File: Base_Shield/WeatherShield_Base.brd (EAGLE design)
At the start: 67.3 x 58.4 mm, 68 parts, among them Q1 BSS138, Q2 BSS138, U1 DS3231SN, U2 LT3652, U3 TMP100MDBVREP, U4 ADS1015IDGST

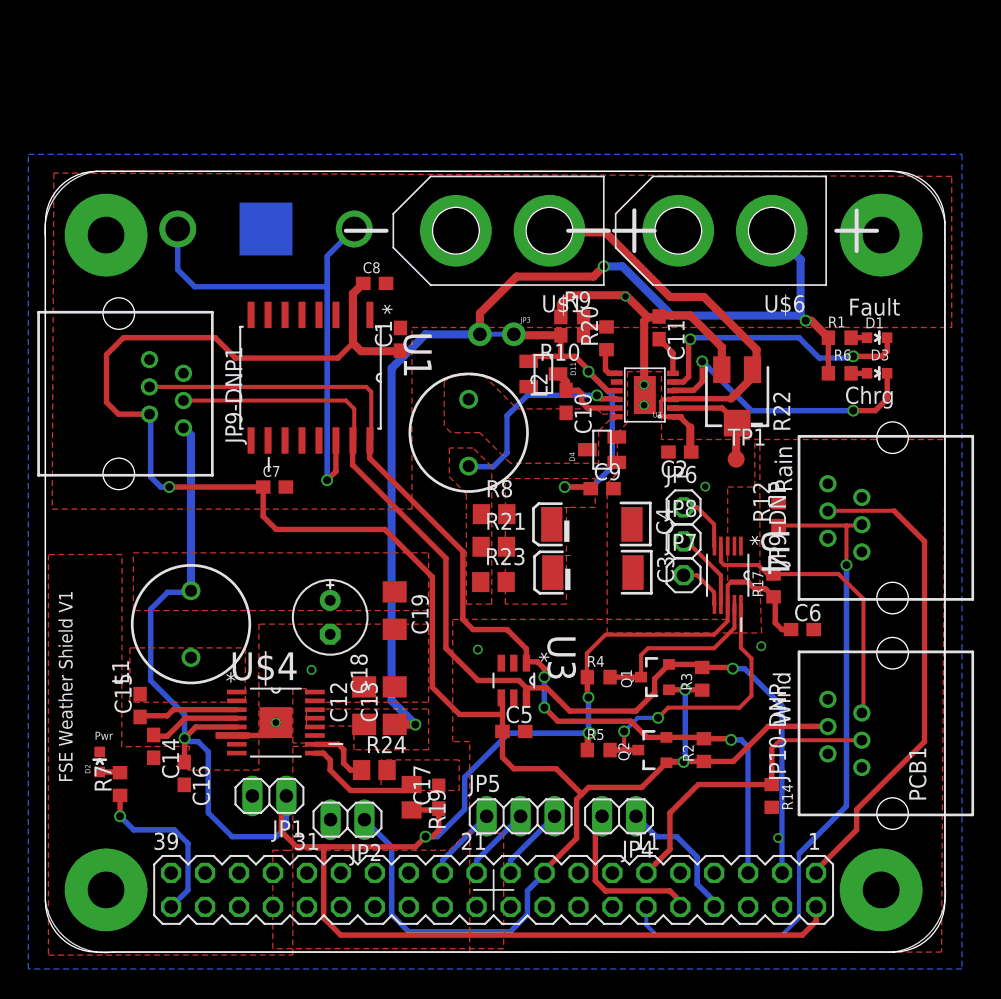
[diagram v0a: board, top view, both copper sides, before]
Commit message: WeatherShield_v1
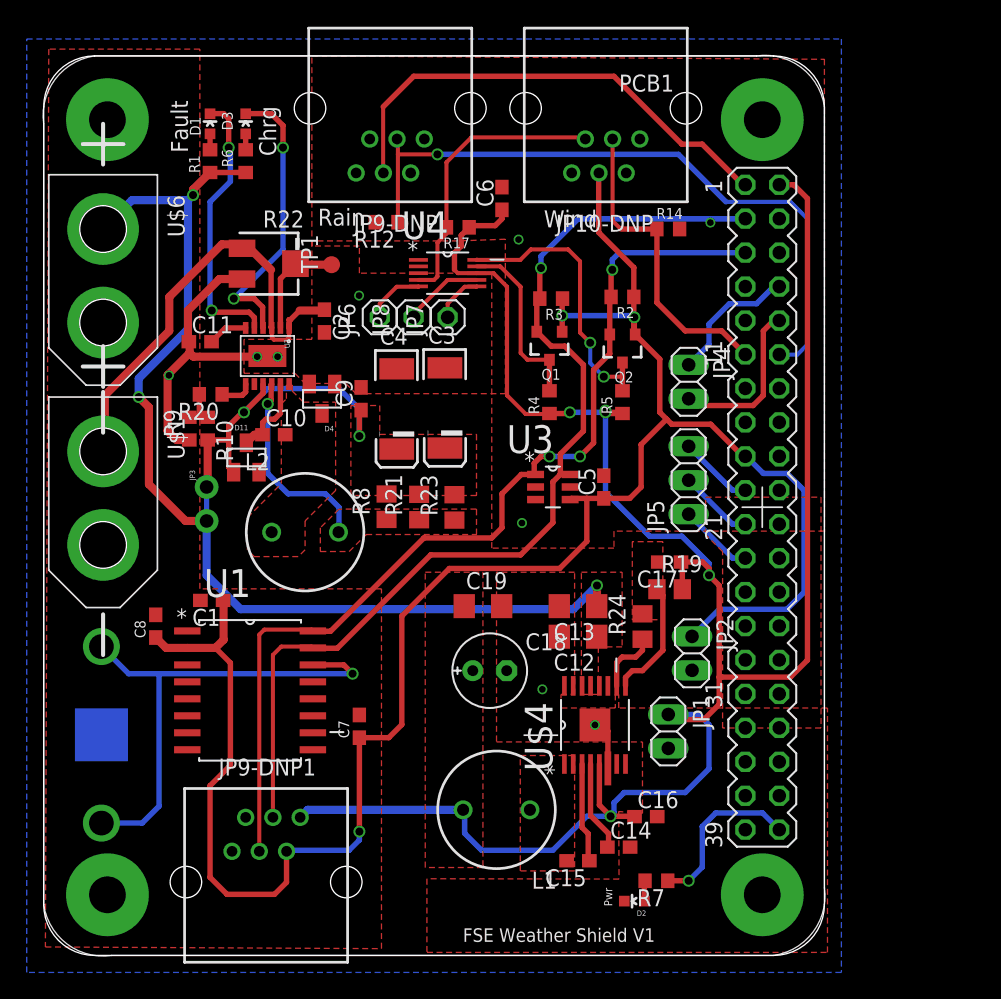
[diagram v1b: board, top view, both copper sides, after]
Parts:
- moved PCB1 68.0 mm to (1.14, 68.3), turned to 270 degrees
- moved JP10-DNP 62.6 mm to (49.3, 70.4), turned to 180 degrees
- moved JP9-DNP 56.9 mm to (33.2, 70.4), turned to 180 degrees
- moved D1 52.4 mm to (13.6, 63.2), turned to 0 degrees
- moved D3 50.8 mm to (16.3, 63.2), turned to 0 degrees
- moved U$6 50.0 mm to (5.59, 55.4), turned to 270 degrees
- moved JP9-DNP1 49.9 mm to (11.7, 0.51), turned to 0 degrees
- moved R1 48.9 mm to (13.6, 60.5), turned to 90 degrees
- moved R6 47.2 mm to (16.3, 60.5), turned to 90 degrees
- moved R14 43.1 mm to (47.9, 55.4), turned to 0 degrees
- moved D2 41.3 mm to (45.3, 5.08), turned to 90 degrees
- moved R7 40.8 mm to (47.0, 6.60), turned to 180 degrees
- moved G1 39.8 mm to (5.46, 17.5), turned to 270 degrees
- moved C6 39.3 mm to (35.4, 57.7), turned to 90 degrees
- moved U$1 37.3 mm to (5.59, 38.7), turned to 270 degrees
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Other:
- board size 67.3 x 58.4 mm -> 58.4 x 67.3 mm
